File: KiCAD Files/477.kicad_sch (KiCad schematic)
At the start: 27 parts, among them IC1 W25N01GVSFIG, IC2 W25N01GVSFIG, IC3 W25N01GVSFIG, IC4 W25N01GVSFIG, J1 BM06B-SRSS-TBT_LF__SN_, J2 6364372-2, J5 BM07B-SRSS-TB_LF__SN_

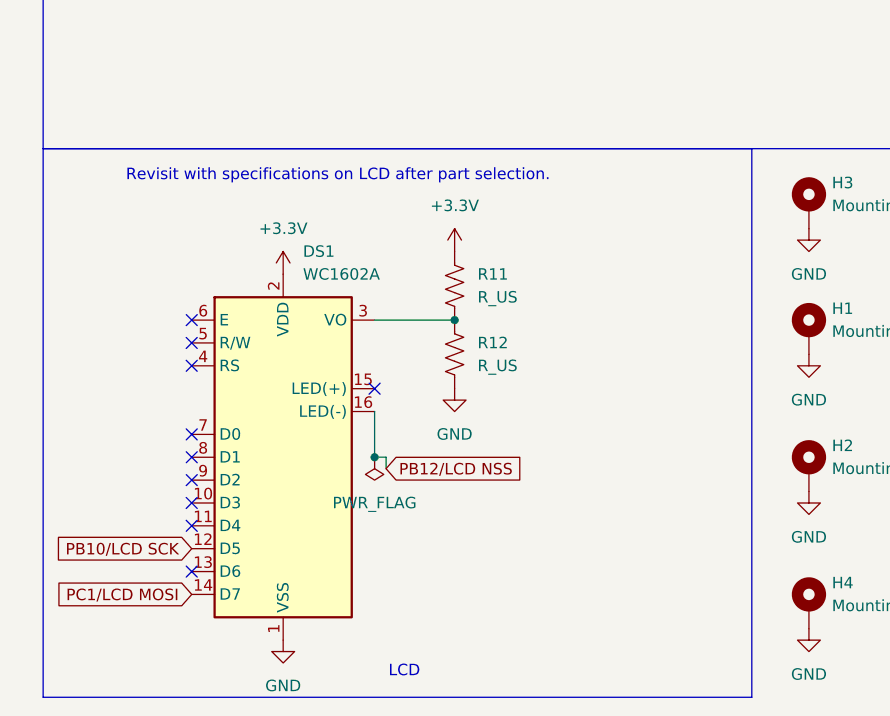
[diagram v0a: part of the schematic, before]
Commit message: found final connector
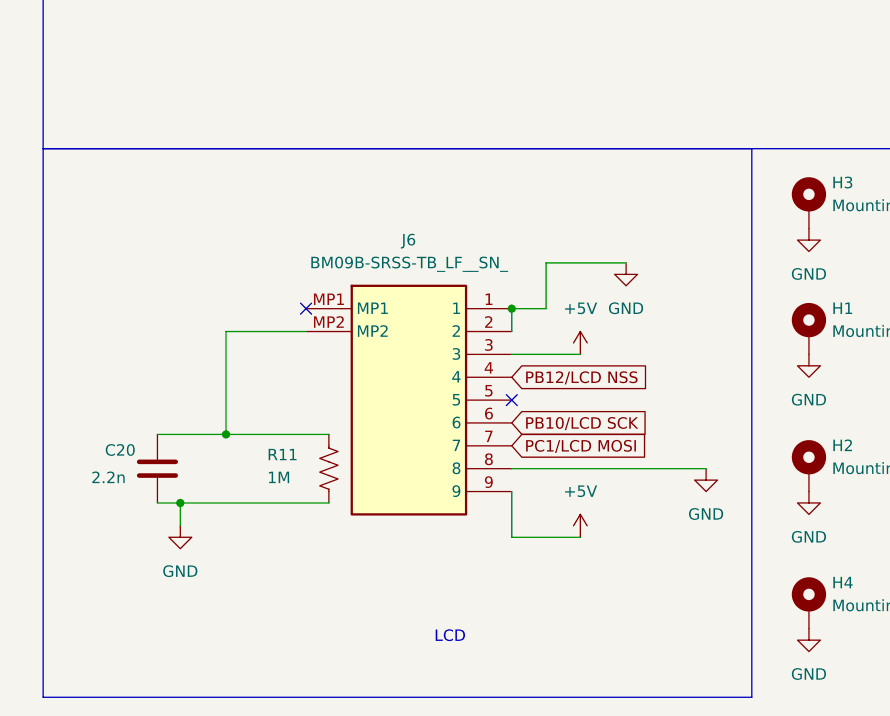
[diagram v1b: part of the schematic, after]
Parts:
- removed DS1: WC1602A, Display:WC1602A, symbol CustomSymbols:WC1602A
- removed R12: R_US, Resistor_SMD:R_0805_2012Metric_Pad1.20x1.40mm_HandSolder, symbol CustomSymbols:R_US
- added C20: 2.2n, Capacitor_SMD:C_0805_2012Metric_Pad1.18x1.45mm_HandSolder, symbol CustomSymbols:C
- added J6: BM09B-SRSS-TB_LF__SN_, BM09BSRSSTBLFSN, symbol CustomSymbols:BM09B-SRSS-TB_LF__SN_
- R11: value R_US -> 1M
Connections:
- net +3.3V: no longer R11.1
- net +5V: now also J6.3, J6.9
- net GND: now also R11.2, C20.2, J6.1, J6.2, J6.8
- net PB10/LCD SCK: now also J6.6
- net PB12/LCD NSS: now also J6.4
- net PC1/LCD MOSI: now also J6.7
- new net: C20.1, J6.MP2, R11.1
- no-connect marks 45 -> 37
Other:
- note removed: "Revisit with specifications on LCD after part selection."
